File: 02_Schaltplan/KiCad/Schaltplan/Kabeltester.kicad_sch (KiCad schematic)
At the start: 12 parts, among them J1 INPUT/MALE-DB9, J14 GND, J15 GND, J16 GND, J2 OUTPUT/FEMALE-DB9, J4 VCC

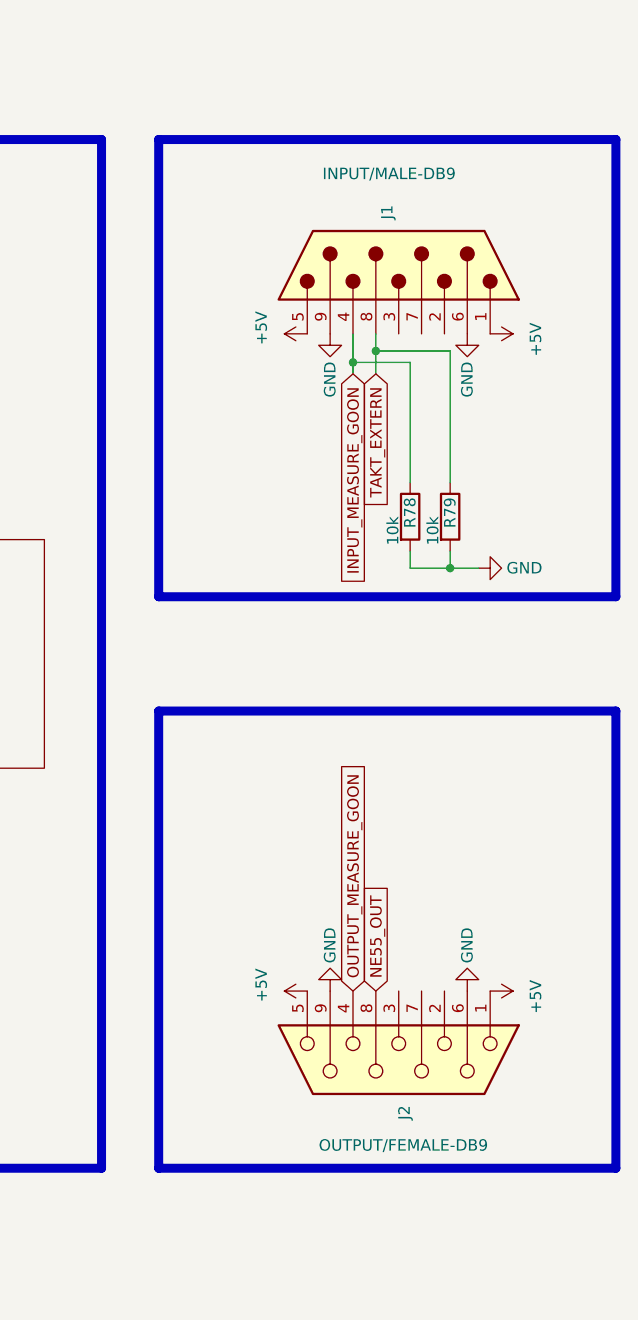
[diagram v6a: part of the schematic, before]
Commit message: Changes
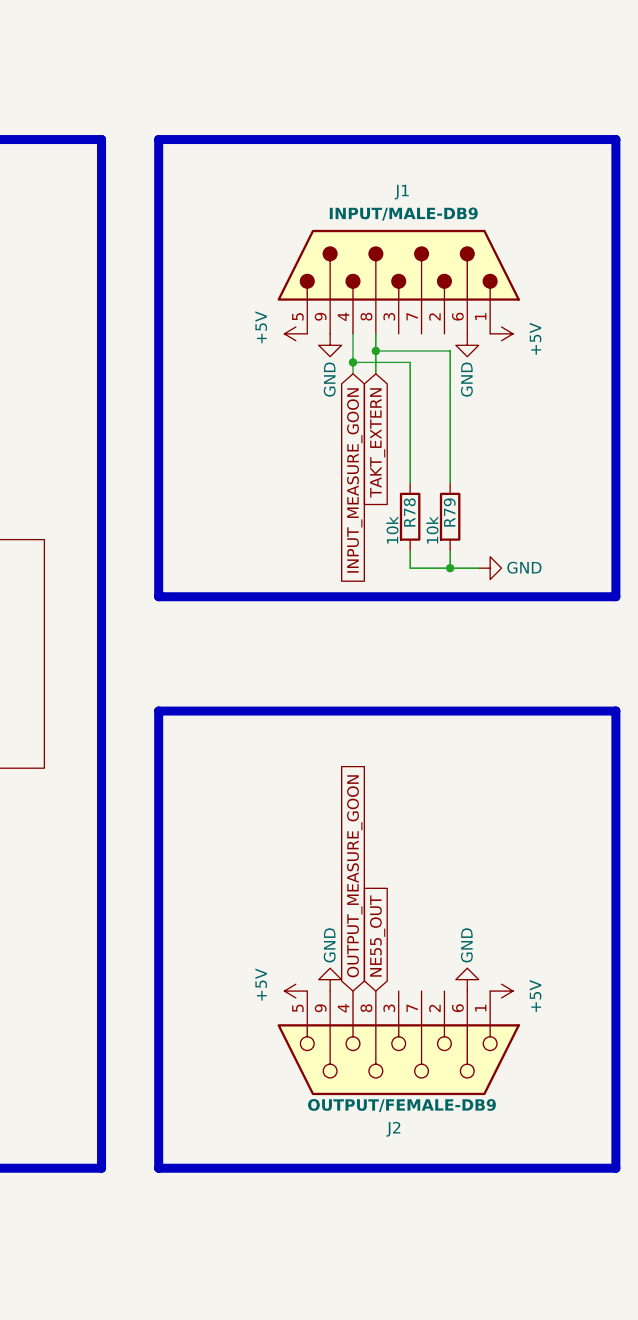
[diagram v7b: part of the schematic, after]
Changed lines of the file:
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@@
   (symbol (lib_id "Connector:DB9_Male") (at 255.27 64.77 90) (unit 1)
     (in_bom yes) (on_board yes)
-    (property "Reference" "J1" (id 0) (at 254 59.69 0)
+    (property "Reference" "J1" (id 0) (at 256.54 56.515 90)
       (effects (font (size 1.27 1.27)) (justify left))
     )
-    (property "Value" "INPUT/MALE-DB9" (id 1) (at 261.62 54.61 90)
-      (effects (font (size 1.27 1.27)) (justify left))
+    (property "Value" "INPUT/MALE-DB9" (id 1) (at 264.16 59.055 90)
+      (effects (font (size 1.27 1.27) bold) (justify left))
     )
     (property "Footprint" "Connector_Dsub:DSUB-9_Male_Horizontal_P2.77x2.84mm_EdgePinOffset4.94mm_Housed_MountingHolesOffset7.48mm" (id 2) (at 255.27 64.77 0)
@@
   (symbol (lib_id "Connector:DB9_Female") (at 255.27 153.035 270) (unit 1)
     (in_bom yes) (on_board yes)
-    (property "Reference" "J2" (id 0) (at 255.905 158.115 0)
+    (property "Reference" "J2" (id 0) (at 254 160.655 90)
       (effects (font (size 1.27 1.27)) (justify left))
     )
-    (property "Value" "OUTPUT/FEMALE-DB9" (id 1) (at 246.38 162.56 90)
-      (effects (font (size 1.27 1.27)) (justify left))
+    (property "Value" "OUTPUT/FEMALE-DB9" (id 1) (at 245.11 158.115 90)
+      (effects (font (size 1.27 1.27) bold) (justify left))
     )
     (property "Footprint" "Connector_Dsub:DSUB-9_Female_Horizontal_P2.77x2.84mm_EdgePinOffset4.94mm_Housed_MountingHolesOffset7.48mm" (id 2) (at 255.27 153.035 0)
